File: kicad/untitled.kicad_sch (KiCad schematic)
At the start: 27 parts, among them J11 Conn_01x02_Socket, J12 Conn_01x02_Socket, J3 AVR-ISP-6, J4 AVR-ISP-6, J5 AVR-ISP-6, J6 Conn_01x01_Pin, J7 Conn_01x01_Pin, J8 Conn_01x01_Pin, J9 Conn_01x01_Pin, M1 Motor_DC, Q1 NMOS, Q2 NMOS, SW4 SW_SPDT, U3 ATmega8A-A, U4 ATmega8A-A, U5 ATmega8A-A

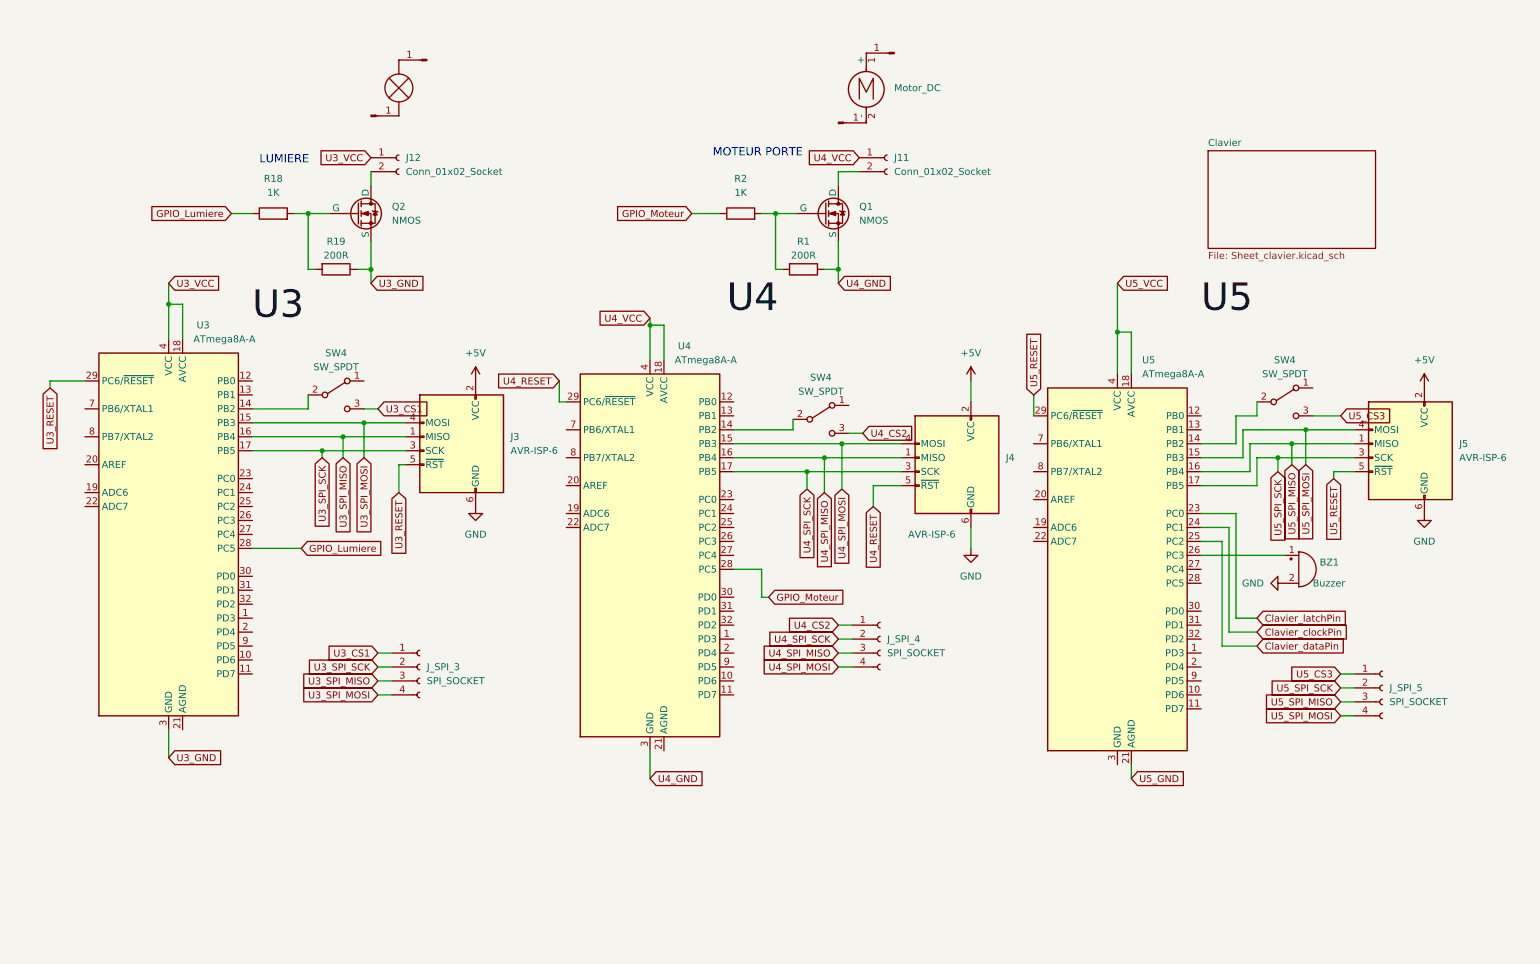
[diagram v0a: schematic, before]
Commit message: kicad update, finalizing
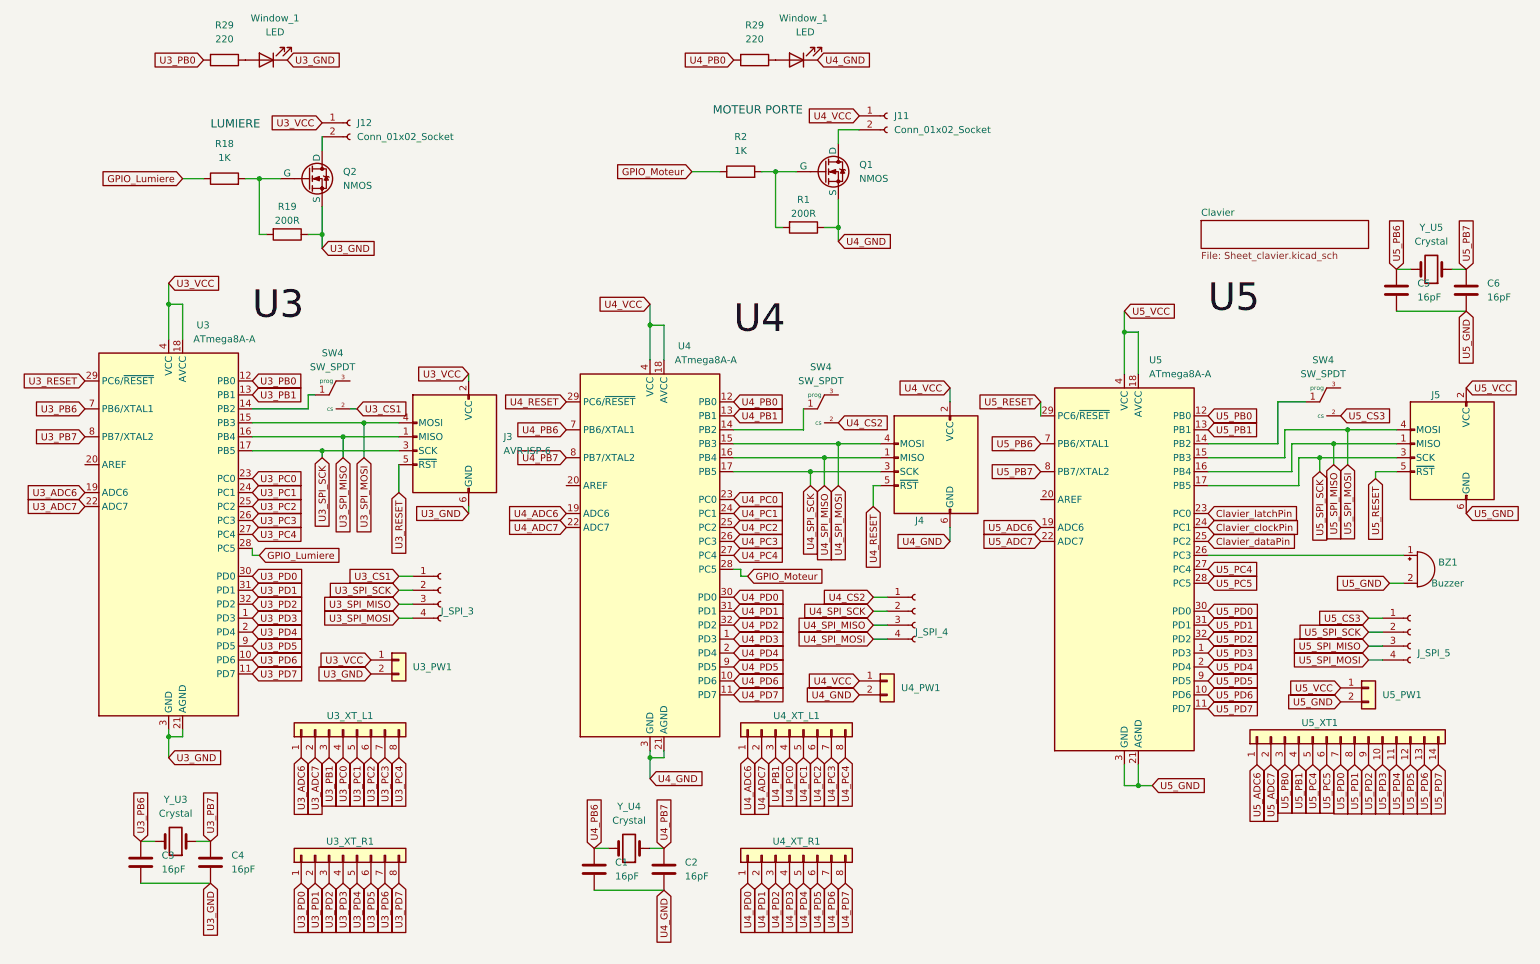
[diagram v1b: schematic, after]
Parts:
- removed J6, J7, J8, J9: Conn_01x01_Pin, symbol Connector:Conn_01x01_Pin
- removed LA1: Lamp, symbol Device:Lamp
- removed M1: Motor_DC, symbol Motor:Motor_DC
- added C1, C2, C3, C4, C5, C6: 16pF, Capacitor_SMD:C_0805_2012Metric_Pad1.18x1.45mm_HandSolder, symbol Device:C
- added R29 (x2): 220, Resistor_SMD:R_0805_2012Metric_Pad1.20x1.40mm_HandSolder, symbol Device:R
- added U3_PW1, U4_PW1, U5_PW1: Conn_01x03_MountingPin, Connector_PinHeader_2.54mm:PinHeader_1x02_P2.54mm_Vertical, symbol Connector_Generic:Conn_01x02
- added U3_XT_L1, U3_XT_R1, U4_XT_L1, U4_XT_R1: Conn_01x08, JP_Library:XT_8, symbol Connector_Generic:Conn_01x08
- added U5_XT1: Conn_01x14, JP_Library:XT_14, symbol Connector_Generic:Conn_01x14
- added Window_1 (x2): LED, LED_SMD:LED_0805_2012Metric, symbol Device:LED
- added Y_U3, Y_U4, Y_U5: Crystal, JP_Library:Crystal 49SS-SMD, symbol Device:Crystal
- J_SPI_5: footprint Connector:NS-Tech_Grove_1x04_P2mm_Vertical -> Connector_PinHeader_2.54mm:PinHeader_1x04_P2.54mm_Vertical
- SW4: footprint JPLibrary:BSI-10 -> JP_Library:BSI-10; symbol Switch:SW_SPDT -> JP_Library:BSI-10
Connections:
- net U3_CS1: now also SW4.2 (cs); no longer SW4.3 (C)
- net U3_GND: now also J3.6 (GND), U3.21 (AGND), C3.2, C4.2, U3_PW1.2 (Pin_2), Window_1.1 (K)
- net U3_VCC: now also J3.2 (VCC), U3_PW1.1 (Pin_1)
- net U4_CS2: now also SW4.2 (cs); no longer SW4.3 (C)
- net U4_GND: now also J4.6 (GND), U4.21 (AGND), C1.2, C2.2, U4_PW1.2 (Pin_2), Window_1.1 (K)
- net U4_VCC: now also J4.2 (VCC), U4_PW1.1 (Pin_1)
- net U5_CS3: now also SW4.2 (cs); no longer SW4.3 (C)
- net U5_GND: now also BZ1.2 (+), J5.6 (GND), U5.3 (GND), U5.5 (GND), C5.2, C6.2, U5_PW1.2 (Pin_2)
- net U5_VCC: now also J5.2 (VCC), U5_PW1.1 (Pin_1)
- net at SW4.1: now also U4.14 (PB2)
- net U5_PD3: now reaches U5.1 (PD3)
- net U5_PD3: now also U5_XT1.10 (Pin_10)
- net U5_PD6: now reaches U5.10 (PD6)
- net U5_PD6: now also U5_XT1.13 (Pin_13)
- net U5_PD7: now reaches U5.11 (PD7)
- net U5_PD7: now also U5_XT1.14 (Pin_14)
- net U5_PB0: now reaches U5.12 (PB0)
- net U5_PB0: now also U5_XT1.3 (Pin_3)
- net U5_PB1: now reaches U5.13 (PB1)
- net U5_PB1: now also U5_XT1.4 (Pin_4)
- net at U5.14 (PB2): now also SW4.1; no longer SW4.2 (B)
- net U5_ADC6: now reaches U5.19 (ADC6)
- net U5_ADC6: now also U5_XT1.1 (Pin_1)
- net U5_PD4: now reaches U5.2 (PD4)
- net U5_PD4: now also U5_XT1.11 (Pin_11)
- net U5_ADC7: now reaches U5.22 (ADC7)
- net U5_ADC7: now also U5_XT1.2 (Pin_2)
- net U5_PC4: now reaches U5.27 (PC4)
- net U5_PC4: now also U5_XT1.5 (Pin_5)
- net U5_PC5: now reaches U5.28 (PC5)
- net U5_PC5: now also U5_XT1.6 (Pin_6)
- net U5_PD0: now reaches U5.30 (PD0)
- net U5_PD0: now also U5_XT1.7 (Pin_7)
- net U5_PD1: now reaches U5.31 (PD1)
- net U5_PD1: now also U5_XT1.8 (Pin_8)
- net U5_PD2: now reaches U5.32 (PD2)
- net U5_PD2: now also U5_XT1.9 (Pin_9)
- net U5_PB6: now reaches U5.7 (PB6/XTAL1)
- net U5_PB6: now also C5.1, Y_U5.2
- net U5_PB7: now reaches U5.8 (PB7/XTAL2)
- net U5_PB7: now also C6.1, Y_U5.1
- net U5_PD5: now reaches U5.9 (PD5)
- net U5_PD5: now also U5_XT1.12 (Pin_12)
- net U3_PD3: now reaches U3.1 (PD3)
- net U3_PD3: now also U3_XT_R1.4 (Pin_4)
- net U3_PD6: now reaches U3.10 (PD6)
- net U3_PD6: now also U3_XT_R1.7 (Pin_7)
- net U3_PD7: now reaches U3.11 (PD7)
- net U3_PD7: now also U3_XT_R1.8 (Pin_8)
- net U3_PB0: now reaches U3.12 (PB0)
- net U3_PB0: now also R29.2
- net U3_PB1: now reaches U3.13 (PB1)
- net U3_PB1: now also U3_XT_L1.3 (Pin_3)
- net at U3.14 (PB2): now also SW4.1; no longer SW4.2 (B)
- net U3_ADC6: now reaches U3.19 (ADC6)
- net U3_ADC6: now also U3_XT_L1.1 (Pin_1)
- net U3_PD4: now reaches U3.2 (PD4)
- net U3_PD4: now also U3_XT_R1.5 (Pin_5)
- net U3_ADC7: now reaches U3.22 (ADC7)
- net U3_ADC7: now also U3_XT_L1.2 (Pin_2)
- net U3_PC0: now reaches U3.23 (PC0)
- net U3_PC0: now also U3_XT_L1.4 (Pin_4)
- net U3_PC1: now reaches U3.24 (PC1)
- net U3_PC1: now also U3_XT_L1.5 (Pin_5)
- net U3_PC2: now reaches U3.25 (PC2)
- net U3_PC2: now also U3_XT_L1.6 (Pin_6)
- net U3_PC3: now reaches U3.26 (PC3)
- net U3_PC3: now also U3_XT_L1.7 (Pin_7)
- net U3_PC4: now reaches U3.27 (PC4)
- net U3_PC4: now also U3_XT_L1.8 (Pin_8)
- net U3_PD0: now reaches U3.30 (PD0)
- net U3_PD0: now also U3_XT_R1.1 (Pin_1)
- net U3_PD1: now reaches U3.31 (PD1)
- net U3_PD1: now also U3_XT_R1.2 (Pin_2)
- net U3_PD2: now reaches U3.32 (PD2)
- net U3_PD2: now also U3_XT_R1.3 (Pin_3)
- net U3_PB6: now reaches U3.7 (PB6/XTAL1)
- net U3_PB6: now also C3.1, Y_U3.2
- net U3_PB7: now reaches U3.8 (PB7/XTAL2)
- net U3_PB7: now also C4.1, Y_U3.1
- net U3_PD5: now reaches U3.9 (PD5)
- net U3_PD5: now also U3_XT_R1.6 (Pin_6)
- net U4_PD3: now reaches U4.1 (PD3)
- net U4_PD3: now also U4_XT_R1.4 (Pin_4)
- net U4_PD6: now reaches U4.10 (PD6)
- net U4_PD6: now also U4_XT_R1.7 (Pin_7)
- net U4_PD7: now reaches U4.11 (PD7)
- net U4_PD7: now also U4_XT_R1.8 (Pin_8)
- net U4_PB0: now reaches U4.12 (PB0)
- net U4_PB0: now also R29.2
- net U4_PB1: now reaches U4.13 (PB1)
- net U4_PB1: now also U4_XT_L1.3 (Pin_3)
- net U4_ADC6: now reaches U4.19 (ADC6)
- net U4_ADC6: now also U4_XT_L1.1 (Pin_1)
- net U4_PD4: now reaches U4.2 (PD4)
- net U4_PD4: now also U4_XT_R1.5 (Pin_5)
- net U4_ADC7: now reaches U4.22 (ADC7)
- net U4_ADC7: now also U4_XT_L1.2 (Pin_2)
- net U4_PC0: now reaches U4.23 (PC0)
- net U4_PC0: now also U4_XT_L1.4 (Pin_4)
- net U4_PC1: now reaches U4.24 (PC1)
- net U4_PC1: now also U4_XT_L1.5 (Pin_5)
- net U4_PC2: now reaches U4.25 (PC2)
- net U4_PC2: now also U4_XT_L1.6 (Pin_6)
- net U4_PC3: now reaches U4.26 (PC3)
- net U4_PC3: now also U4_XT_L1.7 (Pin_7)
- net U4_PC4: now reaches U4.27 (PC4)
- net U4_PC4: now also U4_XT_L1.8 (Pin_8)
- net U4_PD0: now reaches U4.30 (PD0)
- net U4_PD0: now also U4_XT_R1.1 (Pin_1)
- net U4_PD1: now reaches U4.31 (PD1)
- net U4_PD1: now also U4_XT_R1.2 (Pin_2)
- net U4_PD2: now reaches U4.32 (PD2)
- net U4_PD2: now also U4_XT_R1.3 (Pin_3)
- net U4_PB6: now reaches U4.7 (PB6/XTAL1)
- net U4_PB6: now also C1.1, Y_U4.2
- net U4_PB7: now reaches U4.8 (PB7/XTAL2)
- net U4_PB7: now also C2.1, Y_U4.1
- net U4_PD5: now reaches U4.9 (PD5)
- net U4_PD5: now also U4_XT_R1.6 (Pin_6)
- removed net +5V: J3.2 (VCC), J4.2 (VCC), J5.2 (VCC)
- removed net GND: BZ1.2 (+), J3.6 (GND), J4.6 (GND), J5.6 (GND)
- new net: R29.1, Window_1.2 (A) (x2)
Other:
- company: (none) -> JP TOUTANT, JEREMY DIAPHRASE, MOHAND CHAHED
- title: (none) -> SPI SECTION
- moved on the sheet: BZ1, J11, J12, J3, J4, J5, J_SPI_3, J_SPI_4, J_SPI_5, Q1, Q2, R1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

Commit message: switch to SPIs
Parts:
- J3, J4, J5: footprint JPLibrary:SPI_prog -> JP_Library:SPI_prog
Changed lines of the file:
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@@
       (effects (font (size 1.27 1.27)) (justify right) hide)
     )
-    (property "Footprint" "JPLibrary:SPI_prog" (at 278.13 96.52 90)
+    (property "Footprint" "JP_Library:SPI_prog" (at 278.13 96.52 90)
       (effects (font (size 1.27 1.27)) hide)
     )
@@
       (effects (font (size 1.27 1.27)) (justify right))
     )
-    (property "Footprint" "JPLibrary:SPI_prog" (at 96.52 95.25 90)
+    (property "Footprint" "JP_Library:SPI_prog" (at 96.52 95.25 90)
       (effects (font (size 1.27 1.27)) hide)
     )
@@
       (effects (font (size 1.27 1.27)) (justify right) hide)
     )
-    (property "Footprint" "JPLibrary:SPI_prog" (at 184.15 99.06 90)
-      (effects (font (size 1.27 1.27)) hide)
-    )
+    (property "Footprint" "JP_Library:SPI_prog" (at 184.15 99.06 90)
+      (effects (font (size 1.27 1.27)) hide)
+    )
